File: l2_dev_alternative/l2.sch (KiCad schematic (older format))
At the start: 21 parts, among them U301 XS1_L2-QFN124

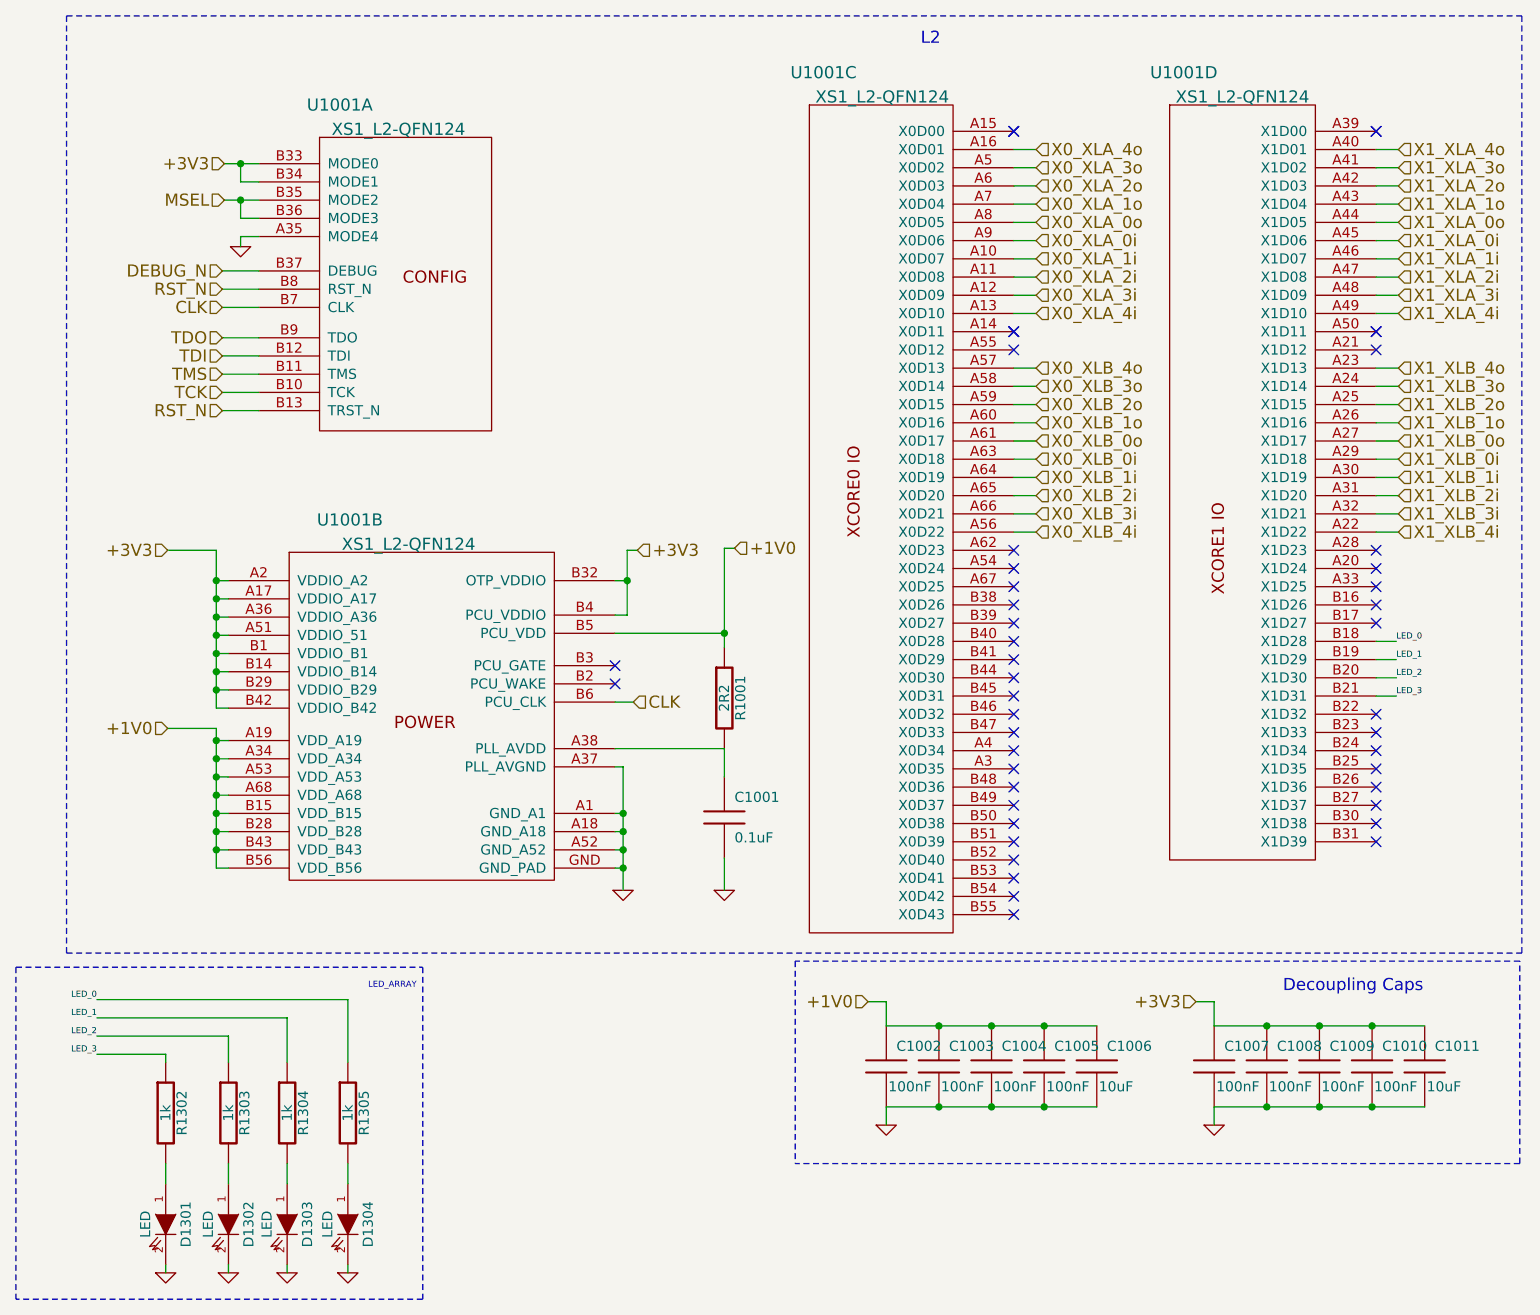
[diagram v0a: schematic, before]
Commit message: done :)
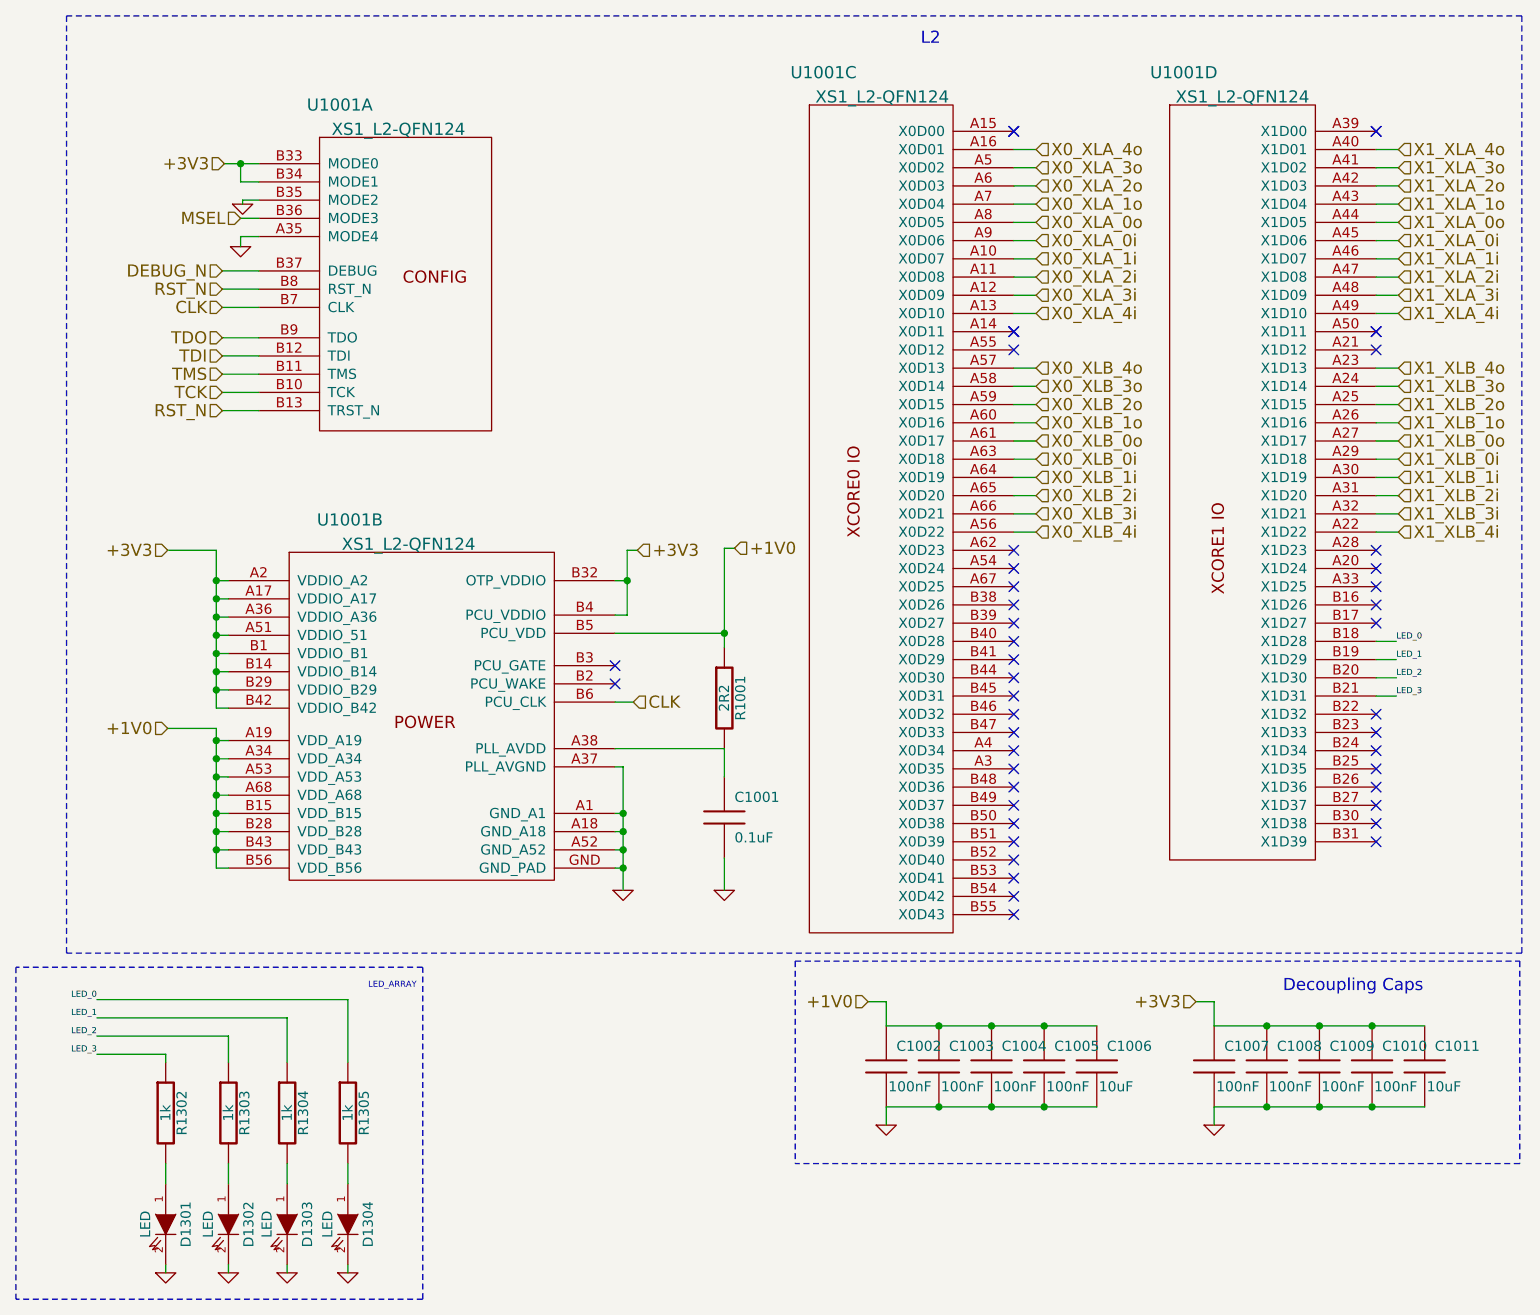
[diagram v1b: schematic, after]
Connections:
- net GND: now also U301.B35 (MODE2)
- net MSEL: no longer U301.B35 (MODE2)
